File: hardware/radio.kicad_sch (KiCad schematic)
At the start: 25 parts, among them J1 105450-0101, J2 Conn_01x02, J3 Conn_01x02, U1 TP4056, U2 ESP32-WROOM-32, U3 TPS5432, U4 MAX98357

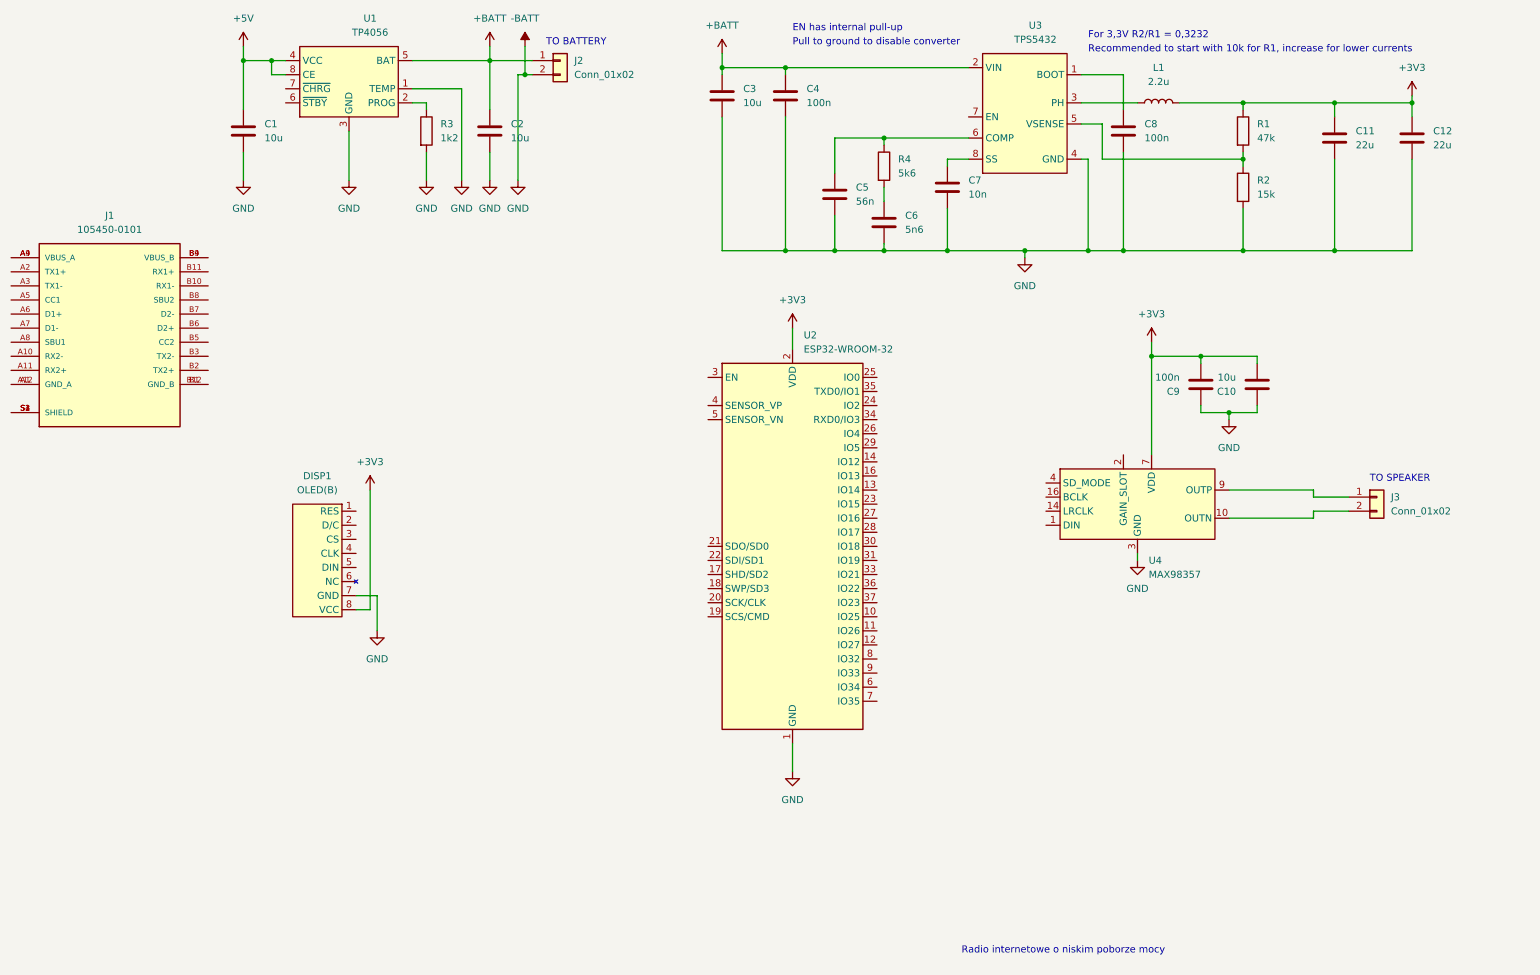
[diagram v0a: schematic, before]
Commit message: schematic
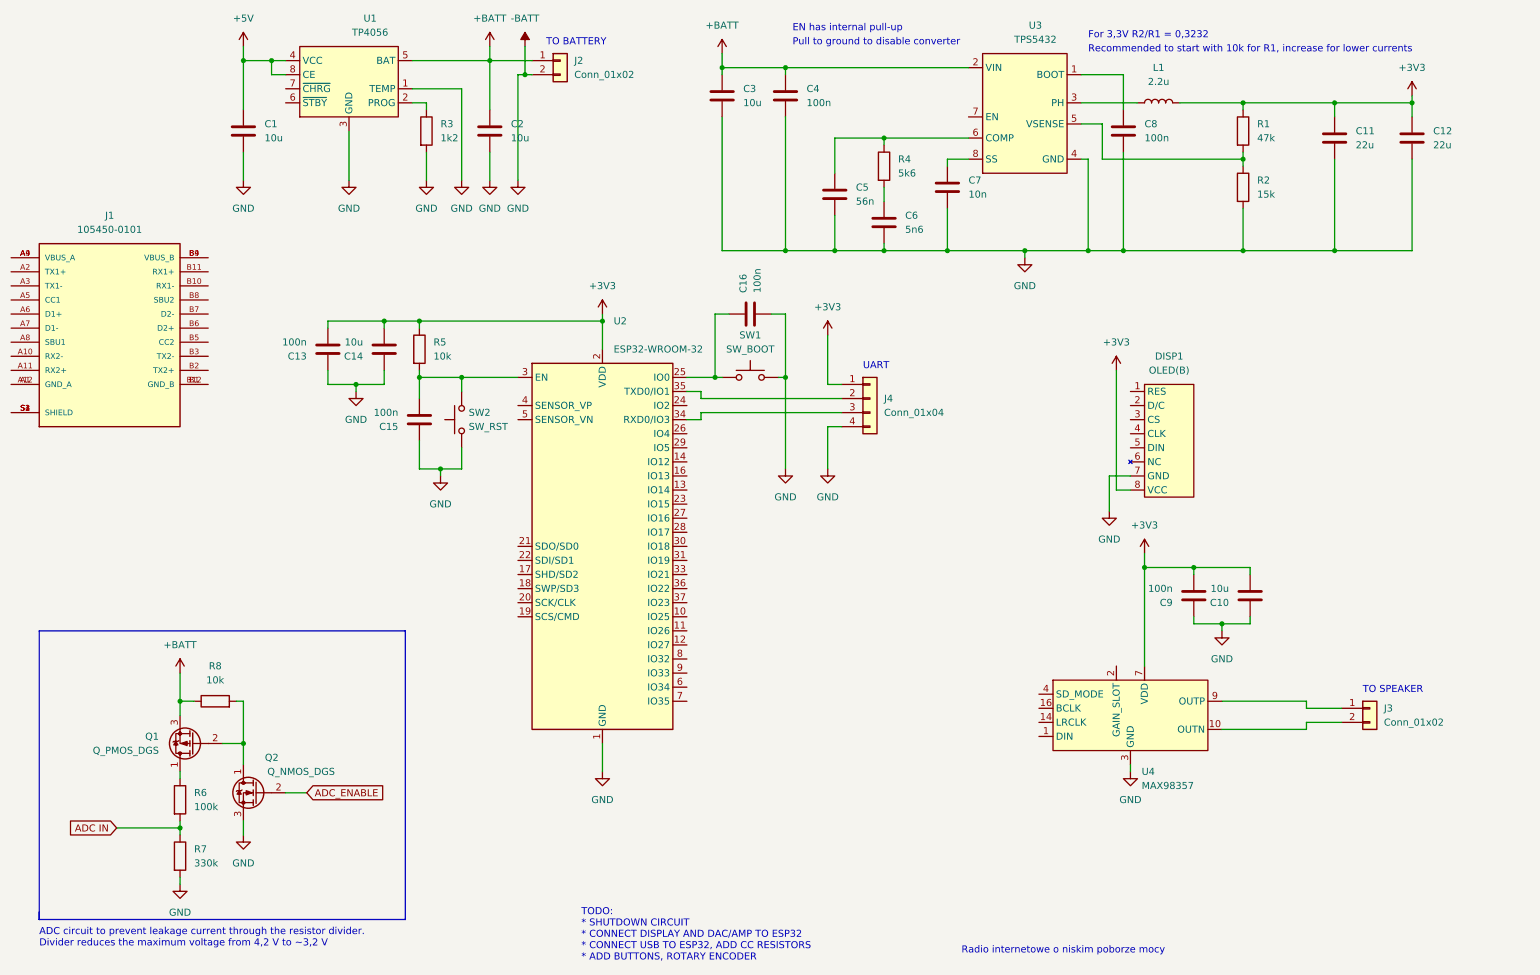
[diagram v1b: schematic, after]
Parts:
- added C13, C15, C16: 100n, Capacitor_SMD:C_0603_1608Metric, symbol Device:C
- added C14: 10u, Capacitor_SMD:C_1206_3216Metric, symbol Device:C
- added J4: Conn_01x04, Connector_PinHeader_2.54mm:PinHeader_1x04_P2.54mm_Vertical, symbol Connector_Generic:Conn_01x04
- added Q1: Q_PMOS_DGS, Package_TO_SOT_SMD:SOT-23, symbol Device:Q_PMOS_DGS
- added Q2: Q_NMOS_DGS, Package_TO_SOT_SMD:SOT-23, symbol Device:Q_NMOS_DGS
- added R5, R8: 10k, Resistor_SMD:R_0603_1608Metric, symbol Device:R
- added R6: 100k, Resistor_SMD:R_0603_1608Metric, symbol Device:R
- added R7: 330k, Resistor_SMD:R_0603_1608Metric, symbol Device:R
- added SW1: SW_BOOT, symbol Switch:SW_Push
- added SW2: SW_RST, symbol Switch:SW_Push
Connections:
- net +3V3: now also C13.2, C14.2, J4.1 (Pin_1), R5.1
- net +BATT: now also Q1.3 (S), R8.1
- net -BATT: now also C13.1, C14.1, C15.1, C16.2, J4.4 (Pin_4), Q2.3 (S), R7.2, SW1.2, SW2.1
- net at U2.25 (IO0): now also C16.1, SW1.1
- net at U2.3 (EN): now also C15.2, R5.2, SW2.2
- net at U2.34 (RXD0/IO3): now also J4.3 (Pin_3)
- net at U2.35 (TXD0/IO1): now also J4.2 (Pin_2)
- new net: Q1.1 (D), R6.1
- new net: Q1.2 (G), Q2.1 (D), R8.2
- new net ADC IN: R6.2, R7.1
- new net ADC_ENABLE: Q2.2 (G)
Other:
- note added: "ADC circuit to prevent leakage current through the resistor divider. Divider reduces the maximum voltage from 4,2 V to ~3,2 V"
- note added: "TODO: * SHUTDOWN CIRCUIT * CONNECT DISPLAY AND DAC/AMP TO ESP32 * CONNECT USB TO ESP32, ADD CC RESISTORS * ADD BUTTONS, ROTARY ENCODER"
- note added: "UART"
- moved on the sheet: C10, C9, DISP1, J3, U2, U4
